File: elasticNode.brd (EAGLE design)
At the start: 160 x 100 mm, 65 parts, among them J1 USB_CONN, U1 PAC1720, U10 FT232R, U2 PAC1720, U4 74AHC573, U5 SST26VF032B, U6 SST26VF032B, U7 LTC3419DFN, U9 MRF24J40MA

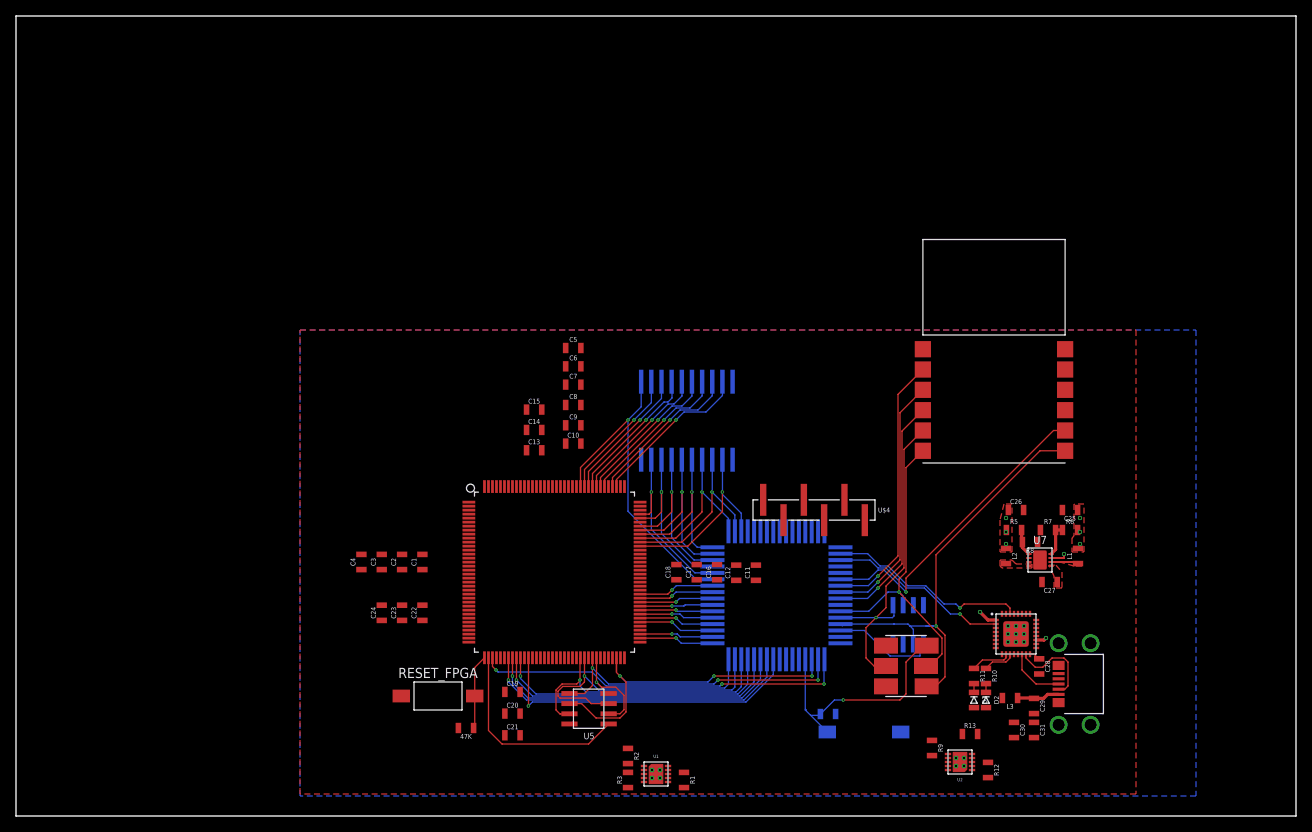
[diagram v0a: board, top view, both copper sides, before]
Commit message: lots of routing, removed latch
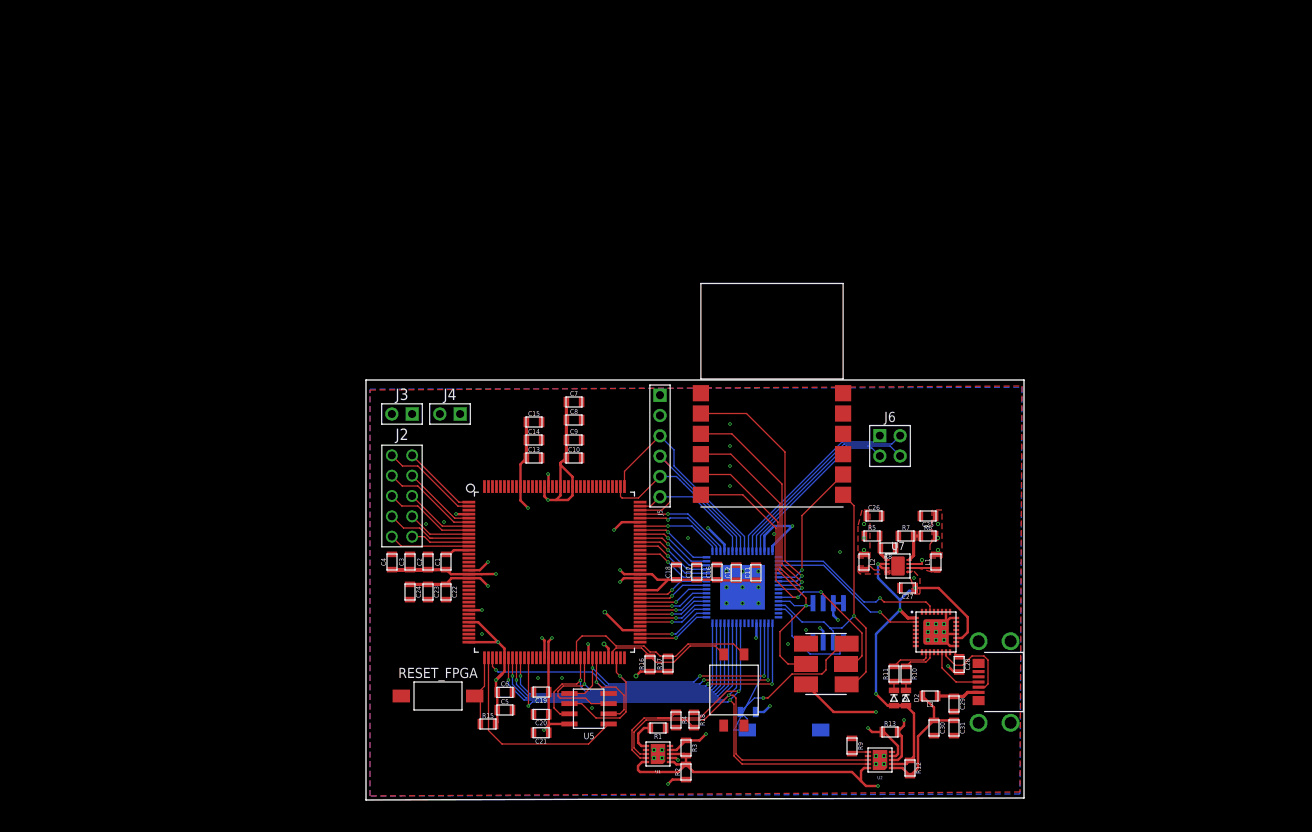
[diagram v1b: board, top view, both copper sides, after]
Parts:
- removed 47K: 15k, passive:0805
- removed U4: 74AHC573, ic:SOIC20
- added J2: FEMALE_HEADER_5X2, connectors:5X2_HEADER
- added J3, J4: FEMALE_HEADER_2X1, connectors:2X1_HEADER
- added J5: JTAG_CONN_6PINTHT, connectors:6X1_HEADER
- added J6: FEMALE_HEADER_2X2, connectors:2X2_HEADER
- added R15: 15k, passive:0805
- added R16, R17: 2.4k, passive:0805
- added R18, R4: 1.5k, passive:0805
- U$1: value ATMEGA64A -> ATMEGA64AQFN; device ic:TQFP64 -> ic:QFN64
- U$4: value FTDI_CONN_6PINSMT_KEEPOUT -> SPST_DIP_2SMT; device connectors:6X1_FTDI_SMT -> connectors:SPST_DIP2_SMT
- moved C5 46.1 mm to (61.1, 13.2)
- moved C6 41.6 mm to (61.1, 15.5)
- moved U9 28.3 mm to (94.5, 46.5)
- moved U$4 24.6 mm to (89.8, 15.8), turned to 0 degrees
- moved C25 17.8 mm to (114.0, 37.5)
- moved C26 17.8 mm to (107.2, 37.5)
- moved L1 17.8 mm to (115.0, 31.8)
- moved L2 17.8 mm to (106.0, 31.8)
- moved R5 17.8 mm to (107.0, 35.0)
- moved R6 17.8 mm to (114.0, 35.0)
- moved R7 17.8 mm to (111.2, 35.0)
- moved R8 17.8 mm to (109.0, 33.5)
- moved U7 17.8 mm to (110.2, 31.2)
- moved C27 17.8 mm to (111.5, 28.5)
- moved C28 10.0 mm to (117.9, 18.9)
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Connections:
- removed net A0: U$2.111, U4.19
- removed net A1: U$2.112, U4.18
- removed net A2: U$2.114, U4.17
- removed net A3: U$2.115, U4.16
- removed net A4: U$2.116, U4.15
- removed net A5: U$2.117, U4.14
- removed net A6: U$2.118, U4.13
- removed net A7: U$2.119, U4.12
- removed net CTS: U$4.2
- removed net FTDI_TXLED: R11.1, U10.10
- removed net N$15: D1.2, R11.2
- removed net N$46: U$2.121
- removed net RTS: U$4.6
- removed net TCK: U$2.109
- removed net TDI: U$2.110
- removed net TDO: U$2.106
- removed net TMS: U$2.107
- new net FPGA_GPIO_0: J2.10, U$2.1
- new net FPGA_GPIO_1: J2.1, U$2.2
- new net FPGA_GPIO_2: J2.9, U$2.5
- new net FPGA_GPIO_3: J2.2, U$2.6
- new net FPGA_GPIO_4: J2.8, U$2.7
- new net FPGA_GPIO_5: J2.3, U$2.8
- new net FPGA_GPIO_6: J2.7, U$2.9
- new net FPGA_GPIO_7: J2.4, U$2.10
- new net FPGA_GPIO_8: J2.6, U$2.11
- new net FPGA_GPIO_9: J2.5, U$2.12
- new net JTAG_TCK: J5.P$3, U$1.57, U$2.109
- new net JTAG_TDI: J5.P$5, U$1.55, U$2.110
- new net JTAG_TDO: J5.P$4, U$1.56, U$2.106
- new net JTAG_TMS: J5.P$6, U$1.54, U$2.107
- new net MCU_GPIO_0: J6.1, U$1.58
- new net MCU_GPIO_1: J6.4, U$1.59
- new net MCU_GPIO_2: J6.3, U$1.60
- new net MCU_GPIO_3: J6.2, U$1.61
- new net N$10: R11.2, U10.10
- new net N$11: D1.2, R11.1
- net 3V3: no longer U$4.3
- net AD0: now also U$2.105; no longer U$2.97, U4.2
- net AD1: now also U$2.104; no longer U$2.98, U4.3
- net AD2: now also U$2.102; no longer U$2.99, U4.4
- net AD3: now also U$2.101; no longer U$2.100, U4.5
- net AD4: now also U$2.100; no longer U$2.101, U4.6
- net AD5: now also U$2.99; no longer U$2.102, U4.7
- net AD6: now also U$2.98; no longer U$2.104, U4.8
- net AD7: now also U$2.97; no longer U$2.105, U4.9
- net ALE: now also U$2.95; no longer U$2.120, U4.11
- net FPGA_RESET: now also R15.1; no longer 47K.1
- net FPGA_VCCAUX: now also J4.1, J5.P$1, R15.2, R16.1, R17.1; no longer 47K.2
- net FPGA_VCCINT: now also J3.1
- net GND: now also J3.3, J4.3, J5.P$2, R18.1, R4.2, U$1.PAD, U$1.VIA1, U$1.VIA2, U$1.VIA3, U$1.VIA4, U$1.VIA5, U$1.VIA6, U$1.VIA7, U$1.VIA8, U$1.VIA9, U$4.3, U$4.4; no longer U$4.1, U4.1, U4.10
- net MCU_RX0: no longer U$2.94, U$4.4
- net MCU_TX0: no longer U$2.95, U$4.5
- net MCU_VCC: no longer U4.20
- net MODE0: now also R16.2, U$4.1
- net MODE1: now also R17.2, U$4.2
- net SELECTMAP_D6/SDA: now also R18.2
- net SELECTMAP_D7/SCL: now also R4.1
- net USB_SHIELD: no longer J1.SHIELD2
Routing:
- net FPGA_VCCAUX: track 0.00 -> 124.0 mm, vias 0 -> 16
- net 3V3: track 2.11 -> 53.2 mm, vias 4 -> 6
- net SELECTMAP_D7/SCL: track 40.2 -> 88.6 mm, vias 1 -> 3
- net 5V: track 4.16 -> 52.1 mm, vias 2 -> 5
- net SELECTMAP_D6/SDA: track 39.7 -> 85.6 mm, vias 1 -> 2
- net FPGA_VCCINT: track 0.00 -> 35.8 mm, vias 0 -> 6
- net ALE: track 41.7 -> 9.50 mm
- net MCU_VCC: track 0.00 -> 29.2 mm, vias 0 -> 7
- net JTAG_TCK: track 0.00 -> 27.0 mm
- net JTAG_TDO: track 0.00 -> 26.5 mm
- net MCU_GPIO_1: track 0.00 -> 25.6 mm
- net MODE1: track 0.00 -> 25.5 mm
- net MCU_GPIO_2: track 0.00 -> 25.1 mm
- net MCU_GPIO_0: track 0.00 -> 23.6 mm
- net JTAG_TDI: track 0.00 -> 22.8 mm
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- added copper zone on layer 3, net FPGA_VCCAUX
- added copper zone on layer 2, net FPGA_VCCINT
- added copper zone on layer 3, net MCU_VCC
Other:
- board size 160 x 100 mm -> 82.2 x 52.5 mm
- board text removed: "analog gnd"

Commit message: added another measurement
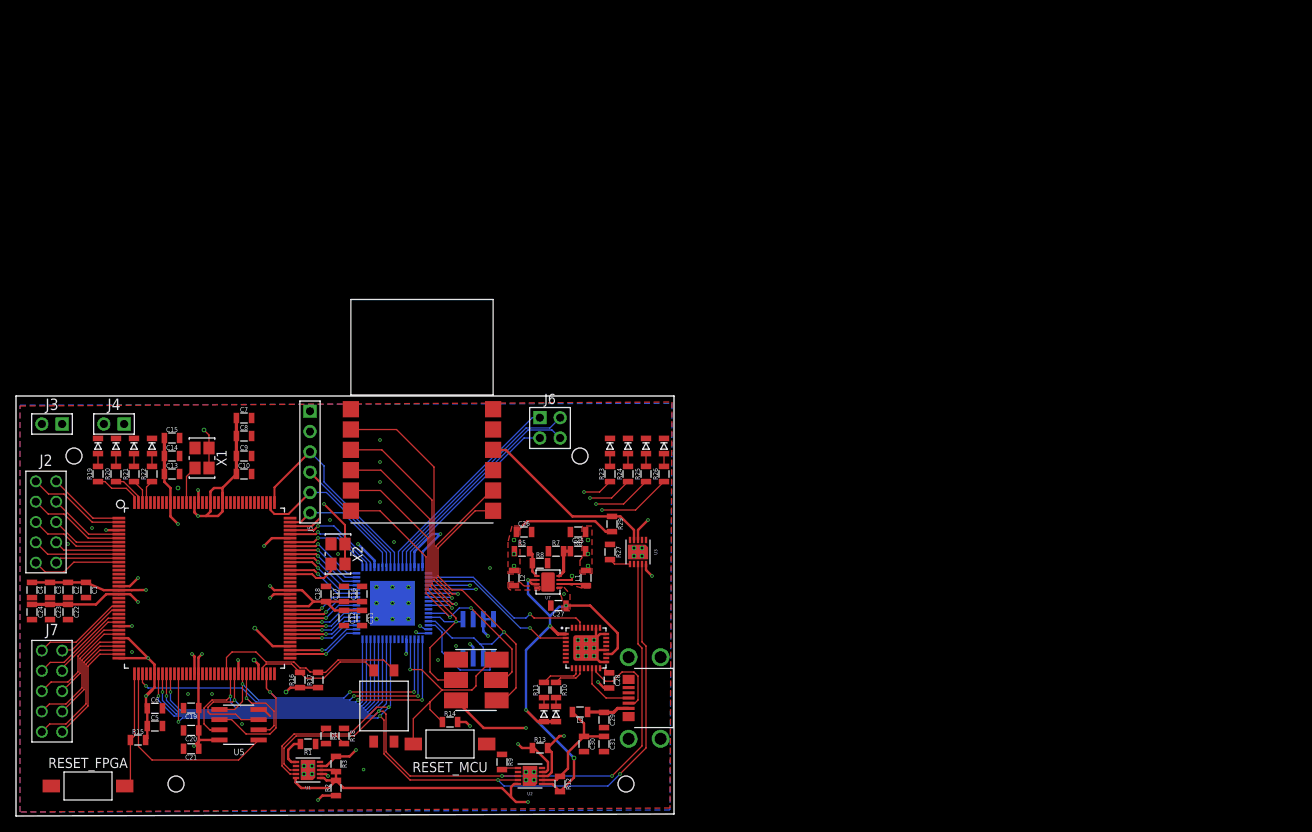
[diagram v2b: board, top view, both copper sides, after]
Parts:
- added D10, D3, D4, D5, D6, D7, D8, D9: (no value), opto:0805
- added J7: FEMALE_HEADER_5X2, connectors:5X2_HEADER
- added R19, R20, R21, R22, R23, R24, R25, R26: (no value), passive:0805
- added R27: 2000, passive:0805
- added R29: 0.5, passive:0805
- added U3: PAC1720, sensors:VDFN10
- added X1: 50MHz, passive:3.2X2.5_OSC
- added X2: 32MHz, passive:3.2X2.5_OSC
- moved C11 49.6 mm to (43.2, 24.8), turned to 270 degrees
- moved C12 49.4 mm to (41.0, 24.8), turned to 270 degrees
- moved C22 47.3 mm to (6.50, 25.5)
- moved C23 47.3 mm to (4.25, 25.5)
- moved C24 47.3 mm to (2.00, 25.5)
- moved C13 45.3 mm to (19.5, 42.8)
- moved C14 45.3 mm to (19.5, 45.0)
- moved C15 45.3 mm to (19.5, 47.2)
- moved RESET_FPGA 45.2 mm to (9.00, 3.75)
- moved C1 45.1 mm to (8.75, 28.2), turned to 270 degrees
- moved C2 45.1 mm to (6.50, 28.2), turned to 270 degrees
- moved C3 45.1 mm to (4.25, 28.2), turned to 270 degrees
- moved C4 45.1 mm to (2.00, 28.2), turned to 270 degrees
- moved J2 44.6 mm to (3.75, 36.8)
- moved C16 44.5 mm to (43.2, 27.8)
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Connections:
- new net FPGA_GPIO_10: J7.10, U$2.24
- new net FPGA_GPIO_11: J7.1, U$2.23
- new net FPGA_GPIO_12: J7.9, U$2.27
- new net FPGA_GPIO_13: J7.2, U$2.26
- new net FPGA_GPIO_14: J7.8, U$2.30
- new net FPGA_GPIO_15: J7.3, U$2.29
- new net FPGA_GPIO_16: J7.7, U$2.33
- new net FPGA_GPIO_17: J7.4, U$2.32
- new net FPGA_GPIO_18: J7.6, U$2.35
- new net FPGA_GPIO_19: J7.5, U$2.34
- new net FPGA_LED0: R19.1, U$2.144
- new net FPGA_LED1: R20.1, U$2.143
- new net FPGA_LED2: R21.1, U$2.142
- new net FPGA_LED3: R22.1, U$2.141
- new net MCU_LED0: R23.1, U$1.16
- new net MCU_LED1: R24.1, U$1.15
- new net MCU_LED2: R25.1, U$1.4
- new net MCU_LED3: R26.1, U$1.5
- new net N$13: D10.1, R26.2
- new net N$15: D9.1, R25.2
- new net N$23: D8.1, R24.2
- new net N$24: D7.1, R23.2
- new net N$25: D6.1, R22.2
- new net N$27: D5.1, R21.2
- new net N$29: D4.1, R20.2
- new net N$30: D3.1, R19.2
- new net N$31: U$2.140
- new net N$32: R27.2, U3.6
- new net OSC_32: U$2.94, X2.3
- new net OSC_50: U$2.131, X1.3
- net 3V3: now also R29.2, U3.10, U3.3
- net 5V: now also R12.2, U2.1; no longer R12.1, U2.2
- net FPGA_VCCAUX: now also X1.1, X1.4, X2.1, X2.4
- net GND: now also D10.2, D3.2, D4.2, D5.2, D6.2, D7.2, D8.2, D9.2, R27.1, R8.2, U3.5, U3.P$1, U3.P$2, U3.P$3, U3.P$4, X1.2, X2.2; no longer R8.1
- net N$2: now also R8.1; no longer R8.2
- net SELECTMAP_D6/SDA: now also U3.8
- net SELECTMAP_D7/SCL: now also U3.9
- net USB_VCC: now also R12.1, U2.2; no longer R12.2, U2.1
- net WIRELESS_VCC: now also R29.1, U3.4
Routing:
- net SELECTMAP_D7/SCL: track 88.6 -> 129.7 mm, vias 3 -> 5
- net SELECTMAP_D6/SDA: track 85.6 -> 125.8 mm, vias 2 -> 4
- net MCU_LED3: track 0.00 -> 37.5 mm, vias 0 -> 2
- net MCU_LED1: track 0.00 -> 36.1 mm, vias 0 -> 2
- net MCU_LED0: track 0.00 -> 35.6 mm, vias 0 -> 2
- net MCU_LED2: track 0.00 -> 34.6 mm, vias 0 -> 2
- net WIRELESS_VCC: track 0.00 -> 23.0 mm
- net FPGA_VCCAUX: track 124.0 -> 141.8 mm, vias 16 -> 18
- net FPGA_GPIO_19: track 0.00 -> 16.8 mm
- net 3V3: track 53.2 -> 69.2 mm, vias 6 -> 8
- net FPGA_GPIO_17: track 0.00 -> 15.3 mm
- net FPGA_GPIO_18: track 0.00 -> 14.0 mm
- net FPGA_GPIO_15: track 0.00 -> 14.0 mm
- net FPGA_GPIO_16: track 0.00 -> 12.5 mm
- net FPGA_GPIO_13: track 0.00 -> 12.4 mm
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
